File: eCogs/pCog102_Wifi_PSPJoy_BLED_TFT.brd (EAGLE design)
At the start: 47.5 x 28 mm, 50 parts, among them T1 MMBT3904LT1G, T3 MMBT3904LT1G, U1 PNA460XM

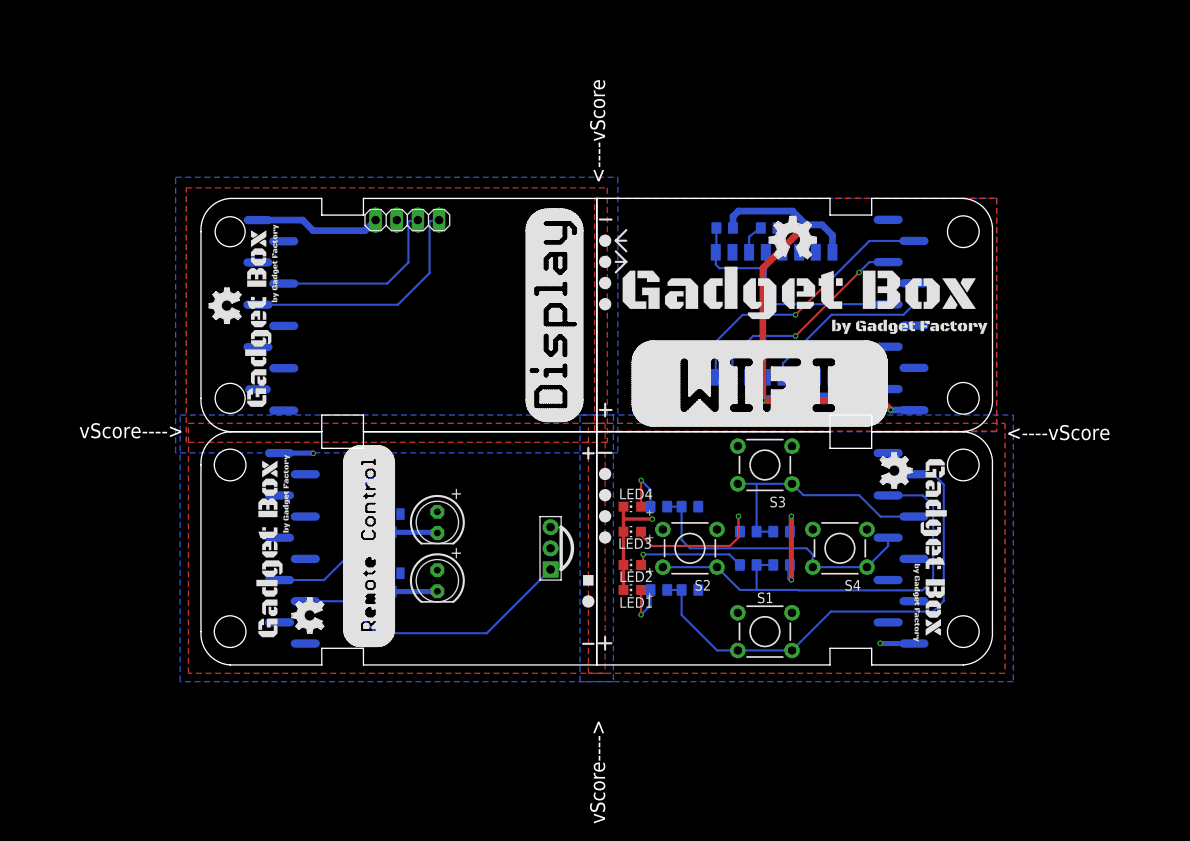
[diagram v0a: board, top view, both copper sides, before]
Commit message: Reorganized
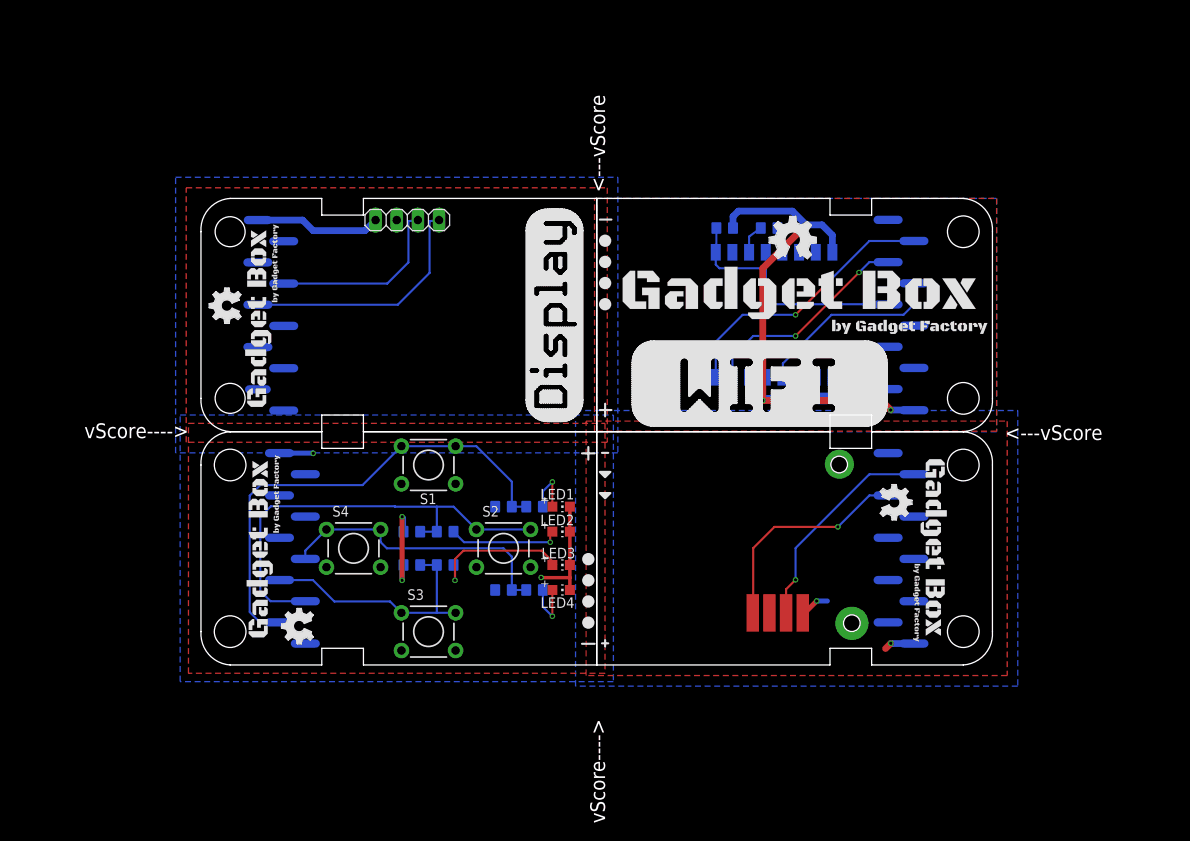
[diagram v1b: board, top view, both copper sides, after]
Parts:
- removed IR1, IR2: (no value), adafruit:LED5MM
- removed R13: 10K, GadgetFactory:0805
- removed T1, T3: MMBT3904LT1G, transistor:SOT23-BEC
- removed U1: PNA460XM, adafruit:PNA460XM
- added U$19: (no value), ohw-logo:OSHW_FILLX200_NOTEXT
- R1: value 1.0 K -> 390; device rcl-ez:R0805 -> GadgetFactory:0805
- R2, R4, R6, R8: value 390 -> 10K
- R3, R5, R7: value 10K -> 390
- U$10, U$12: device ohw-logo:OSHW_FILLX150_NOTEXT -> GadgetFactory:GADGETBOX_SMALL
- U$11: device GadgetFactory:GADGETBOX_SMALL -> ohw-logo:OSHW_FILLX150_NOTEXT
- U$13: device GadgetFactory:GADGETBOX_TEXT -> ohw-logo:OSHW_FILLX150_NOTEXT
- U$14: device eCogs:LEGEND_DIO -> GadgetFactory:GADGETBOX_TEXT
- U$18: device ohw-logo:OSHW_FILLX200_NOTEXT -> eCogs:LEGEND_DIO
- U$2: device eCogs:LEGEND_PWM -> eCogs:LEGEND_DIO
- U$7: value (none) -> JOYSTICK-PSP1000; device eCogs:LEGEND_DIO -> SparkFun:JOYSTICK-PSP1000
- U$8: device eCogs:LEGEND_DIO -> eCogs:LEGEND_ANALOG
- U$9: device GadgetFactory:GADGETBOX_SMALL -> eCogs:LEGEND_ANALOG
- moved U$11 77.2 mm to (82.0, 21.6), turned to 270 degrees
- moved U$13 67.2 mm to (5.29, 41.0), turned to 90 degrees
- moved S4 58.4 mm to (18.8, 14.0), turned to 0 degrees
- moved S3 45.1 mm to (27.8, 4.00), turned to 0 degrees
- moved S1 45.1 mm to (27.8, 24.0), turned to 0 degrees
- moved R6 40.6 mm to (25.8, 12.0), turned to 180 degrees
- moved R4 40.6 mm to (25.8, 16.0), turned to 180 degrees
- moved R5 40.4 mm to (29.8, 12.0), turned to 180 degrees
- moved U$9 39.9 mm to (49.0, 20.4), turned to 180 degrees
- moved R7 30.5 mm to (40.5, 9.00), turned to 180 degrees
- moved R3 30.2 mm to (29.8, 16.0), turned to 180 degrees
- moved R11 24.1 mm to (63.4, 52.4), turned to 180 degrees
- moved U$14 23.4 mm to (72.4, 44.4), turned to 0 degrees
- moved S2 22.4 mm to (36.8, 14.0), turned to 0 degrees
- moved U$7 21.7 mm to (69.7, 14.0)
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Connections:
- removed net BLAST_RX: ECOG.G0
- removed net BLAST_TX: ECOG.G3
- removed net N$12: R13.1, X1.3
- removed net N$7 (its old number): IR1.K, T1.C
- removed net N$8 (its old number): R10.1, X1.11
- removed net RECEIVE: ECOG.G1, U1.1
- removed net TRANSMIT: ECOG.G2, R1.1
- new net HORIZONTAL: ECOG1.G1, U$7.X
- new net VERTICAL: ECOG1.G0, U$7.Y
- net 1: now also ECOG.G0, R1.1, R2.2; no longer ECOG1.G0, R2.1, R3.2
- net 2: now also ECOG.G1, R3.1, R4.2; no longer ECOG1.G1, R4.1, R5.2
- net 3: now also ECOG.G2, R5.1, R6.2; no longer ECOG1.G2, R6.1, R7.2
- net 3V3: now also R11.2, R9.2, U$7.VCC; no longer IR1.A, IR2.A, R10.2, R13.2, U1.3
- net 4: now also ECOG.G3, R7.1, R8.2; no longer ECOG1.G3, R8.1, R9.2
- net GND: now also R10.1, R2.1, R4.1, R6.1, R8.1, U$7.GND; no longer R11.1, R3.1, R5.1, R7.1, R9.1, T1.E, T3.E, U1.2
- net N$1: now also R1.2; no longer R2.2
- net N$10: now also R10.2, X1.10; no longer R1.2, T1.B, T3.B
- net N$11: now also R12.1, X1.3; no longer R11.2, X1.10
- net N$2: now also R3.2; no longer R4.2
- net N$3: now also R5.2; no longer R6.2
- net N$4: now also R7.2; no longer R8.2
- net N$9: now also R9.1, X1.11; no longer IR2.K, T3.C
- net RESET: now also R11.1; no longer R12.1
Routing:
- net RECEIVE: track 34.2 -> 0.00 mm
- net HORIZONTAL: track 0.00 -> 26.6 mm, vias 0 -> 1
- net VERTICAL: track 0.00 -> 26.1 mm, vias 0 -> 1
- net TRANSMIT: track 21.6 -> 0.00 mm
- net N$10: track 9.72 -> 2.90 mm
- net N$7 (its old number): track 5.39 -> 0.00 mm
- net N$12: track 3.63 -> 0.00 mm
- net GND: track 24.8 -> 28.4 mm, vias 3 -> 4
- net N$9: track 5.41 -> 2.56 mm
- net N$8 (its old number): track 2.56 -> 0.00 mm
- net N$11: track 2.90 -> 3.63 mm
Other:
- board text added: "<---vScore"
- board text added: "Horizontal"
- board text added: "PSP Thumb Joystick"
- board text added: "Vert"
- board text added: "XC0"
- board text added: "XC1"
- board text added: "XC2"
- board text added: "XC3"
- board text added: "ecog104 v2.0"
- board text added: "ecog104.GadgetFactory.net"
- board text removed: "+"
- board text removed: "0"
- board text removed: "1"
- board text removed: "2"
- board text removed: "3"
- board text removed: "<----vScore"
- board text removed: "RECEIVE"
- board text removed: "Remote Control"
- board text removed: "TRANSMIT"
- board text removed: "ecog107 v2.0"
- board text removed: "ecog107.GadgetFactory.net"
